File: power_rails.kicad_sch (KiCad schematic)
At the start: 30 parts, among them SW3 ~{SR}, SW4 ~{PB}, U12 MCP1799T-5002H/TT, U5 AP63200WU, U7 AP63205WU, U8 STM6601CM2DDM6F, U9 TPS62162DSG

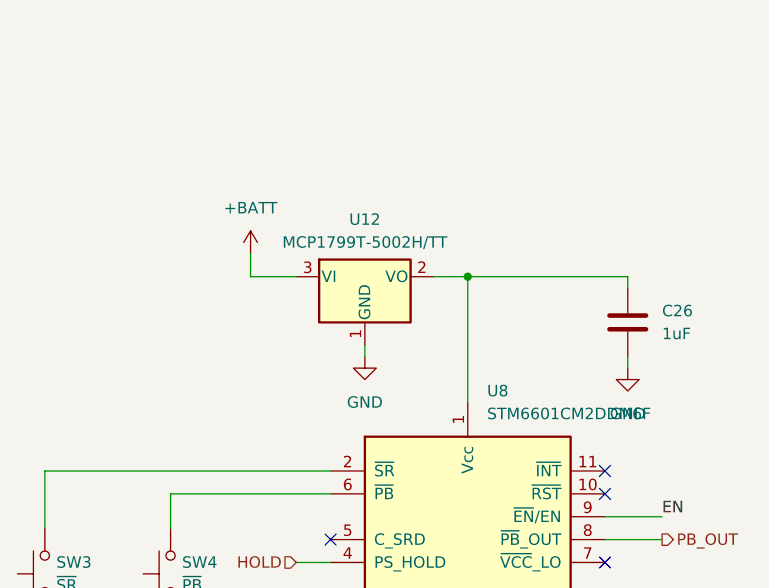
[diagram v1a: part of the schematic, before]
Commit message: finalized component selection
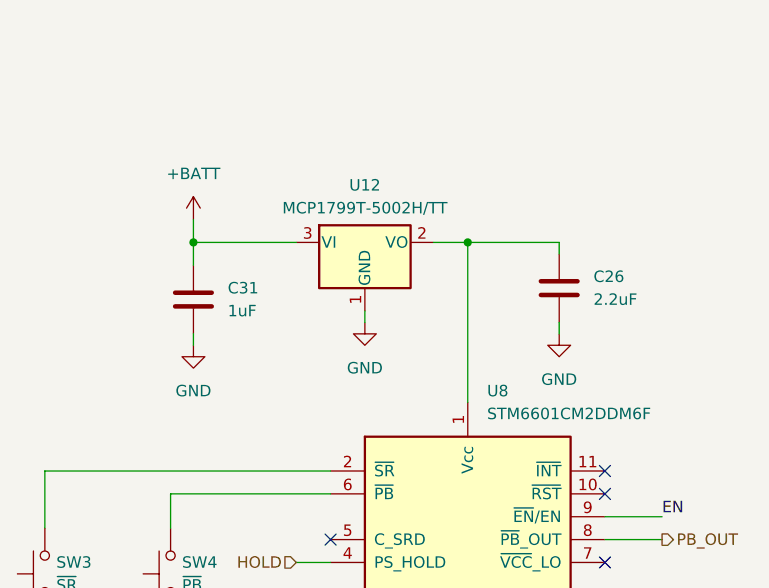
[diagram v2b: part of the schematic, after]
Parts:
- added C31: 1uF, Capacitor_SMD:C_0603_1608Metric, symbol Device:C
- C26: value 1uF -> 2.2uF; LCSC C5673 -> C415535; MPN CL10A105KA8NNNC -> (none); Manufacturer Samsung Electro-Mechanics -> (none)
- L2: footprint Inductor_SMD:L_APV_ANR3012 -> Inductor_SMD:L_Coilcraft_LPS3010
- L3: footprint Inductor_SMD:L_Sunlord_MWSA0503S -> Inductor_SMD:L_Chilisin_BWVS00505030
- L4: LCSC C431344 -> C408412; MPN CMLW5040S100MST -> (none); Manufacturer Cybermax -> Sunlord
- R12: LCSC C2906982 -> C15401; MPN FRC0603F1002TS -> (none); Manufacturer FOJAN -> UNI-ROYAL(Uniroyal Elec)
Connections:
- net +BATT: now also C31.1
- net GND: now also C31.2
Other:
- moved on the sheet: C26, U12

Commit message: add MPS entries
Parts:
- C13, C19: MPN CC0603KRX7R9BB104 -> GPN; Manufacturer YAGEO -> Generic
- C17, C20, C21, C23, C24, C28: MPN CL21A226KOQNNNE -> GPN; Manufacturer Samsung Electro-Mechanics -> Generic
- C18, C22, C25: MPN GRM21BR61E106KA73L -> GPN; Manufacturer muRata -> Generic
- C26, C31: MPN (none) -> GPN; Manufacturer (none) -> Generic
- C32: MPN CL10A105KA8NNNC -> GPN; Manufacturer Samsung Electro-Mechanics -> Generic
- D3: MPN KT-0603R -> 150060RS75000; Manufacturer Hubei KENTO Elec -> Wurth Elektronik
- R11: MPN 0603WAF6492T5E -> GPN; Manufacturer UNI-ROYAL -> Generic
- R12: MPN (none) -> GPN; Manufacturer UNI-ROYAL(Uniroyal Elec) -> Generic
- R15: MPN 0603WAF1003T5E -> GPN; Manufacturer UNI-ROYAL -> Generic
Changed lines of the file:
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@@
 			)
 		)
-		(property "Manufacturer" "Samsung Electro-Mechanics"
+		(property "Manufacturer" "Generic"
 			(at 0 0 0)
 			(hide yes)
@@
 			)
 		)
-		(property "MPN" "CL21A226KOQNNNE"
+		(property "MPN" "GPN"
 			(at 0 0 0)
 			(hide yes)
@@
 			)
 		)
+		(property "Manufacturer" "Generic" (at 0 0 0)
+			(effects
+				(font
+					(size 1.27 1.27)
+				)
+				(hide yes)
+			)
+		)
+		(property "MPN" "GPN" (at 0 0 0)
+			(effects
+				(font
+					(size 1.27 1.27)
+				)
+				(hide yes)
+			)
+		)
 		(pin "1"
 		)
@@
 			)
 		)
-		(property "Manufacturer" "Samsung Electro-Mechanics"
+		(property "Manufacturer" "Generic"
 			(at 0 0 0)
 			(hide yes)
@@
 			)
 		)
-		(property "MPN" "CL21A226KOQNNNE"
+		(property "MPN" "GPN"
 			(at 0 0 0)
 			(hide yes)
@@
 			)
 		)
-		(property "Manufacturer" "UNI-ROYAL"
+		(property "Manufacturer" "Generic"
 			(at 0 0 0)
 			(hide yes)
@@
 			)
 		)
-		(property "MPN" "0603WAF6492T5E"
+		(property "MPN" "GPN"
 			(at 0 0 0)
 			(hide yes)
@@
 			)
 		)
-		(property "Manufacturer" "Samsung Electro-Mechanics"
+		(property "Manufacturer" "Generic"
 			(at 0 0 0)
 			(hide yes)
@@
 			)
 		)
-		(property "MPN" "CL21A226KOQNNNE"
+		(property "MPN" "GPN"
 			(at 0 0 0)
 			(hide yes)
@@
 			)
 		)
-		(property "Manufacturer" "YAGEO"
+		(property "Manufacturer" "Generic"
 			(at 0 0 0)
 			(hide yes)
@@
 			)
 		)
-		(property "MPN" "CC0603KRX7R9BB104"
+		(property "MPN" "GPN"
 			(at 0 0 0)
 			(hide yes)
@@
 			)
 		)
-		(property "Manufacturer" "YAGEO"
+		(property "Manufacturer" "Generic"
 			(at 0 0 0)
 			(hide yes)
@@
 			)
 		)
-		(property "MPN" "CC0603KRX7R9BB104"
+		(property "MPN" "GPN"
 			(at 0 0 0)
 			(hide yes)
@@
 			)
 		)
-		(property "Manufacturer" "Samsung Electro-Mechanics"
+		(property "Manufacturer" "Generic"
 			(at 0 0 0)
 			(hide yes)
@@
 			)
 		)
-		(property "MPN" "CL21A226KOQNNNE"
+		(property "MPN" "GPN"
 			(at 0 0 0)
 			(hide yes)
@@
 			)
 		)
-		(property "Manufacturer" "muRata"
+		(property "Manufacturer" "Generic"
 			(at 0 0 0)
 			(hide yes)
@@
 			)
 		)
-		(property "MPN" "GRM21BR61E106KA73L"
+		(property "MPN" "GPN"
 			(at 0 0 0)
 			(hide yes)
@@
 			)
 		)
-		(property "Manufacturer" "Samsung Electro-Mechanics"
+		(property "Manufacturer" "Generic"
 			(at 0 0 0)
 			(hide yes)
@@
 			)
 		)
-		(property "MPN" "CL21A226KOQNNNE"
+		(property "MPN" "GPN"
 			(at 0 0 0)
 			(hide yes)
@@
 			)
 		)
-		(property "Manufacturer" "muRata"
+		(property "Manufacturer" "Generic"
 			(at 0 0 0)
 			(hide yes)
@@
 			)
 		)
-		(property "MPN" "GRM21BR61E106KA73L"
+		(property "MPN" "GPN"
 			(at 0 0 0)
 			(hide yes)
@@
 			)
 		)
-		(property "Manufacturer" "UNI-ROYAL(Uniroyal Elec)"
+		(property "Manufacturer" "Generic"
 			(at 0 0 0)
 			(hide yes)
@@
 			)
 		)
-		(property "MPN" ""
+		(property "MPN" "GPN"
 			(at 0 0 0)
 			(hide yes)
@@
 			)
 		)
-		(property "MPN" ""
+		(property "MPN" "GPN"
 			(at -7.62 -3.81 0)
 			(hide yes)
@@
 			)
 		)
-		(property "Manufacturer" ""
+		(property "Manufacturer" "Generic"
 			(at -7.62 -3.81 0)
 			(hide yes)
@@
 			)
 		)
-		(property "Manufacturer" "Samsung Electro-Mechanics"
+		(property "Manufacturer" "Generic"
 			(at 0 0 0)
 			(hide yes)
@@
 			)
 		)
-		(property "MPN" "CL21A226KOQNNNE"
+		(property "MPN" "GPN"
 			(at 0 0 0)
 			(hide yes)
@@
 			)
 		)
-		(property "Manufacturer" "UNI-ROYAL"
+		(property "Manufacturer" "Generic"
 			(at 0 0 0)
 			(hide yes)
@@
 			)
 		)
-		(property "MPN" "0603WAF1003T5E"
+		(property "MPN" "GPN"
 			(at 0 0 0)
 			(hide yes)
@@
 			)
 		)
-		(property "Manufacturer" "Hubei KENTO Elec"
+		(property "Manufacturer" "Wurth Elektronik"
 			(at 0 0 0)
 			(hide yes)
@@
 			)
 		)
-		(property "MPN" "KT-0603R"
+		(property "MPN" "150060RS75000"
 			(at 0 0 0)
 			(hide yes)
@@
 			)
 		)
-		(property "Manufacturer" "muRata"
+		(property "Manufacturer" "Generic"
 			(at 0 0 0)
 			(hide yes)
@@
 			)
 		)
-		(property "MPN" "GRM21BR61E106KA73L"
+		(property "MPN" "GPN"
 			(at 0 0 0)
 			(hide yes)
@@
 			)
 		)
-		(property "MPN" "CL10A105KA8NNNC"
+		(property "MPN" "GPN"
 			(at 0 0 0)
 			(hide yes)
@@
 			)
 		)
-		(property "Manufacturer" "Samsung Electro-Mechanics"
+		(property "Manufacturer" "Generic"
 			(at 0 0 0)
 			(hide yes)

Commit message: update MPN codes
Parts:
- C13, C19: MPN GPN -> GPC0603104
- C17, C20, C21, C23, C24, C28: MPN GPN -> GPC0805226
- C18, C22, C25: MPN GPN -> GPC0805106
- C26: MPN GPN -> GPC0603225
- C31, C32: MPN GPN -> GPC0603105
- R11: MPN GPN -> GPR0603649
- R12: MPN GPN -> GPR060310K
- R15: MPN GPN -> GPR0603100K
- TP1, TP2, TP3: now left out of the parts list
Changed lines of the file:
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@@
 			)
 		)
-		(property "MPN" "GPN"
+		(property "MPN" "GPC0805226"
 			(at 0 0 0)
 			(hide yes)
@@
 			)
 		)
-		(property "Manufacturer" "Generic" (at 0 0 0)
+		(property "Manufacturer" "Generic"
+			(at 0 0 0)
+			(hide yes)
+			(show_name no)
+			(do_not_autoplace no)
 			(effects
 				(font
 					(size 1.27 1.27)
 				)
-				(hide yes)
 			)
 		)
-		(property "MPN" "GPN" (at 0 0 0)
+		(property "MPN" "GPC0603105"
+			(at 0 0 0)
+			(hide yes)
+			(show_name no)
+			(do_not_autoplace no)
 			(effects
 				(font
 					(size 1.27 1.27)
 				)
-				(hide yes)
 			)
 		)
@@
 		(body_style 1)
 		(exclude_from_sim no)
-		(in_bom yes)
+		(in_bom no)
 		(on_board yes)
 		(in_pos_files yes)
@@
 			)
 		)
-		(property "MPN" "GPN"
+		(property "MPN" "GPC0805226"
 			(at 0 0 0)
 			(hide yes)
@@
 			)
 		)
-		(property "MPN" "GPN"
+		(property "MPN" "GPR0603649"
 			(at 0 0 0)
 			(hide yes)
@@
 			)
 		)
-		(property "MPN" "GPN"
+		(property "MPN" "GPC0805226"
 			(at 0 0 0)
 			(hide yes)
@@
 			)
 		)
-		(property "MPN" "GPN"
+		(property "MPN" "GPC0603104"
 			(at 0 0 0)
 			(hide yes)
@@
 			)
 		)
-		(property "MPN" "GPN"
+		(property "MPN" "GPC0603104"
 			(at 0 0 0)
 			(hide yes)
@@
 		(body_style 1)
 		(exclude_from_sim no)
-		(in_bom yes)
+		(in_bom no)
 		(on_board yes)
 		(in_pos_files yes)
@@
 			)
 		)
-		(property "MPN" "GPN"
+		(property "MPN" "GPC0805226"
 			(at 0 0 0)
 			(hide yes)
@@
 			)
 		)
-		(property "MPN" "GPN"
+		(property "MPN" "GPC0805106"
 			(at 0 0 0)
 			(hide yes)
@@
 			)
 		)
-		(property "MPN" "GPN"
+		(property "MPN" "GPC0805226"
 			(at 0 0 0)
 			(hide yes)
@@
 			)
 		)
-		(property "MPN" "GPN"
+		(property "MPN" "GPC0805106"
 			(at 0 0 0)
 			(hide yes)
@@
 			)
 		)
-		(property "MPN" "GPN"
+		(property "MPN" "GPR060310K"
 			(at 0 0 0)
 			(hide yes)
@@
 		(body_style 1)
 		(exclude_from_sim no)
-		(in_bom yes)
+		(in_bom no)
 		(on_board yes)
 		(in_pos_files yes)
@@
 			)
 		)
-		(property "MPN" "GPN"
+		(property "MPN" "GPC0603225"
 			(at -7.62 -3.81 0)
 			(hide yes)
@@
 			)
 		)
-		(property "MPN" "GPN"
+		(property "MPN" "GPC0805226"
 			(at 0 0 0)
 			(hide yes)
@@
 			)
 		)
-		(property "MPN" "GPN"
+		(property "MPN" "GPR0603100K"
 			(at 0 0 0)
 			(hide yes)
@@
 			)
 		)
-		(property "MPN" "GPN"
+		(property "MPN" "GPC0805106"
 			(at 0 0 0)
 			(hide yes)
@@
 			)
 		)
-		(property "MPN" "GPN"
+		(property "MPN" "GPC0603105"
 			(at 0 0 0)
 			(hide yes)
